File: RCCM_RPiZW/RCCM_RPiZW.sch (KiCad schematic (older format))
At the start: 31 parts, among them CN1 Conn_02x20_Odd_Even, CN2 Conn_02x04_Odd_Even, CN3 Conn_01x08, CN4 Conn_01x06, CN5 Conn_01x07, CN6 Conn_01x06, IC1 LP2950-3.0_TO92, J1 Conn_01x02, J2 Conn_01x02

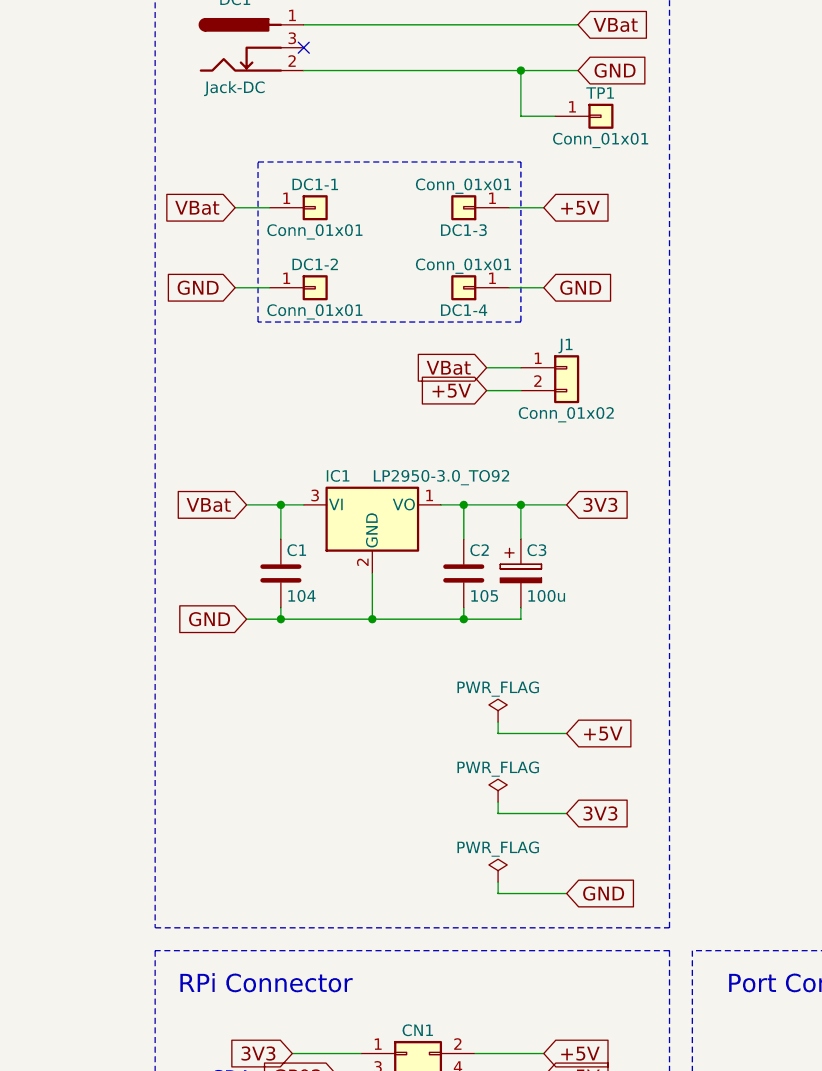
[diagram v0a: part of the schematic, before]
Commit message: Update RPiZW Gerber
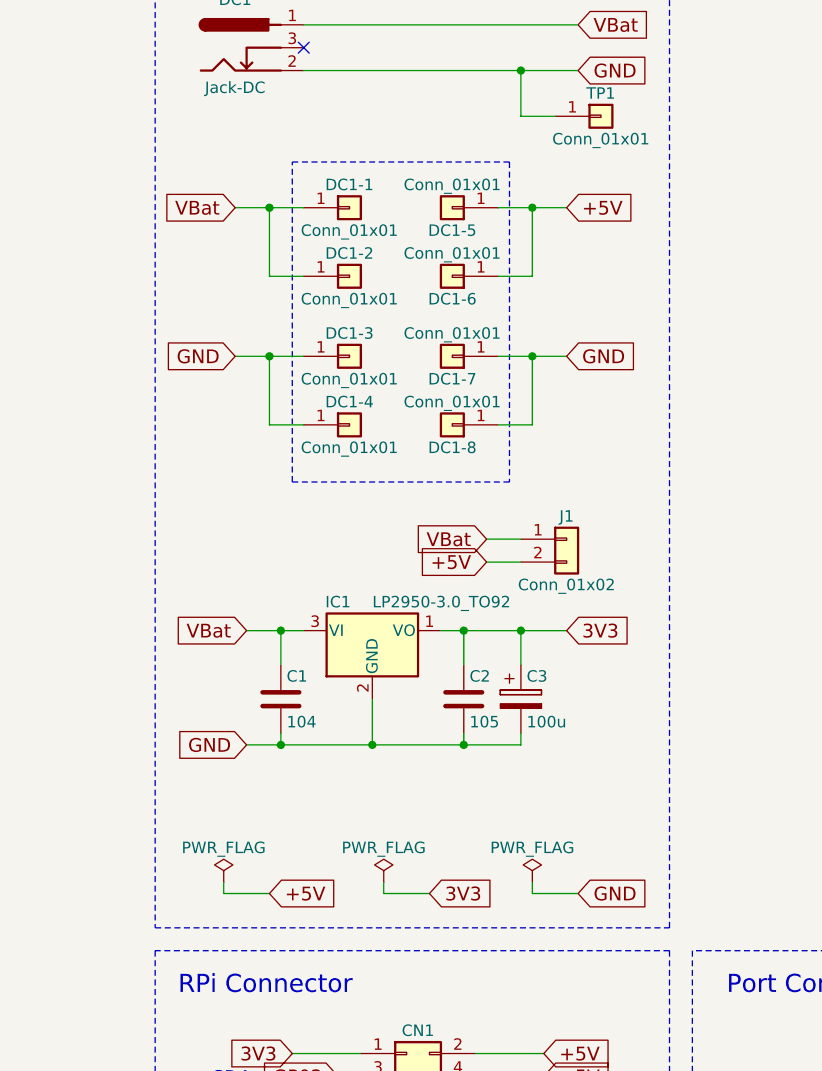
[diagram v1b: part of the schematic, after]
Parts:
- added DC1-3, DC1-6, DC1-7, DC1-8: Conn_01x01, Pin_Headers:Pin_Header_Straight_1x01_Pitch2.54mm, symbol Conn_01x01
- renumbered DC1-3 to DC1-5
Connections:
- net +5V: now also DC1-6.1 (Pin_1)
- net GND: now also DC1-3.1 (Pin_1), DC1-7.1 (Pin_1), DC1-8.1 (Pin_1); no longer DC1-2.1 (Pin_1)
- net VBat: now also DC1-2.1 (Pin_1)
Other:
- moved on the sheet: C1, C2, C3, DC1-1, DC1-5, IC1, J1
